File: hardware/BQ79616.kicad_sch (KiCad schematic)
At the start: 9 parts, among them CN7 4x100nF, IC2 BQ79616PAPR

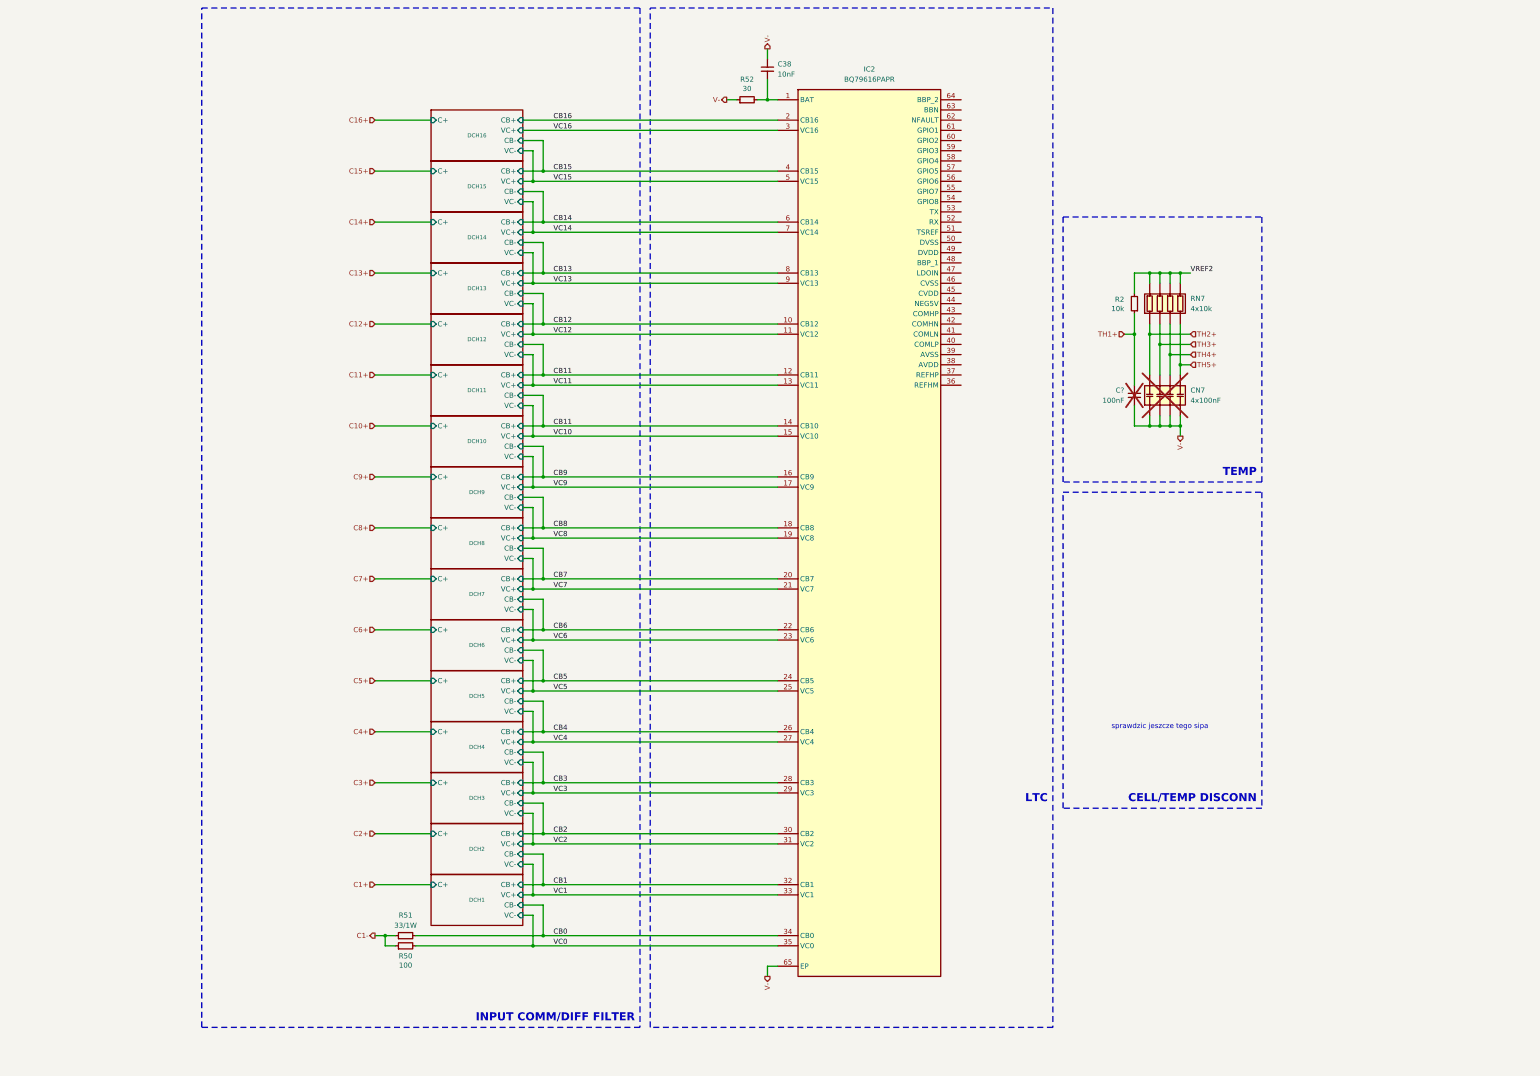
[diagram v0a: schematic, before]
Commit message: sync
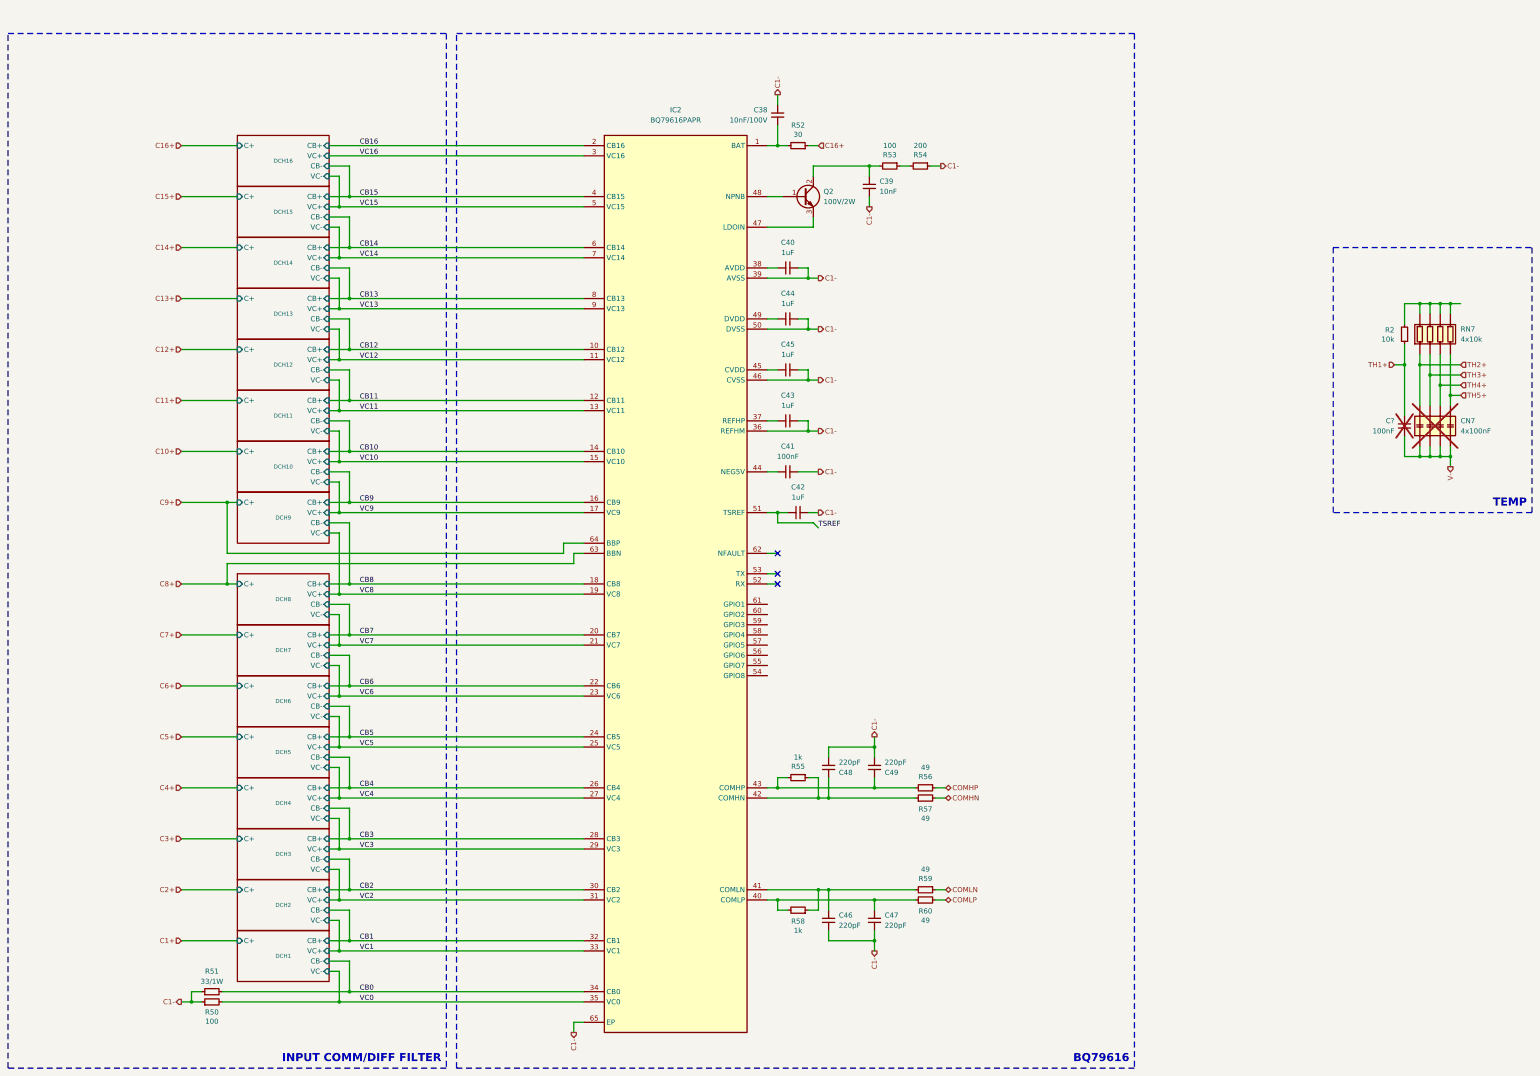
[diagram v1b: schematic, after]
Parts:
- added C39: 10nF, Capacitor_SMD:C_0603_1608Metric, symbol Device:C_Small
- added C40, C42, C43, C44, C45: 1uF, Capacitor_SMD:C_0603_1608Metric, symbol Device:C_Small
- added C41: 100nF, Capacitor_SMD:C_0603_1608Metric, symbol Device:C_Small
- added C46, C47, C48, C49: 220pF, Capacitor_SMD:C_0603_1608Metric, symbol Device:C_Small
- added Q2: 100V/2W, Package_TO_SOT_SMD:SOT-223-3_TabPin2, symbol Device:Q_NPN_BCE
- added R53: 100, Resistor_SMD:R_0603_1608Metric, symbol PUTM_EV_BMS_HV_Slave_2021-rescue:R_Small-Device
- added R54: 200, Resistor_SMD:R_0603_1608Metric, symbol PUTM_EV_BMS_HV_Slave_2021-rescue:R_Small-Device
- added R55, R58: 1k, Resistor_SMD:R_0603_1608Metric, symbol PUTM_EV_BMS_HV_Slave_2021-rescue:R_Small-Device
- added R56, R57, R59, R60: 49, Resistor_SMD:R_0603_1608Metric, symbol PUTM_EV_BMS_HV_Slave_2021-rescue:R_Small-Device
- C38: value 10nF -> 10nF/100V
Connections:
- net C1-: now also C38.1, IC2.36 (REFHM), IC2.39 (AVSS), IC2.46 (CVSS), IC2.50 (DVSS), IC2.65 (EP), C39.2, C40.2, C41.2, C42.2, C43.2, C44.2, C45.2, C46.2, C47.2, C48.2, C49.2, R54.1
- net C16+: now also R52.1
- net C8+: now also IC2.63 (BBN)
- net C9+: now also IC2.64 (BBP)
- net CB11: no longer IC2.14 (CB10)
- net V-: no longer C38.1, IC2.65 (EP), R52.1
- net at IC2.37 (REFHP): now also C43.1
- net at IC2.38 (AVDD): now also C40.1
- net at IC2.40 (COMLP): now also C47.1, R58.2, R60.1
- net at IC2.41 (COMLN): now also C46.1, R58.1, R59.2
- net at IC2.42 (COMHN): now also C48.1, R55.1, R57.1
- net at IC2.43 (COMHP): now also C49.1, R55.2, R56.2
- net at IC2.44 (NEG5V): now also C41.1
- net at IC2.45 (CVDD): now also C45.1
- net at IC2.47 (LDOIN): now also Q2.3 (E)
- net at IC2.48 (NPNB): now also Q2.1 (B)
- net at IC2.49 (DVDD): now also C44.1
- net TSREF: now reaches IC2.51 (TSREF)
- net TSREF: now also C42.1
- net VREF2: no longer names the net of R2.2, RN7.5 (R4.2), RN7.6 (R3.2), RN7.7 (R2.2), RN7.8 (R1.2)
- new net: C39.1, Q2.2 (C), R53.2
- new net: R53.1, R54.2
- new net CB10: IC2.14 (CB10)
- new net COMHN: R57.2
- new net COMHP: R56.1
- new net COMLN: R59.1
- new net COMLP: R60.2
- no-connect marks 0 -> 3
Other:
- note added: "BQ79616"
- note removed: "CELL/TEMP DISCONN"
- note removed: "LTC"
- note removed: "sprawdzic jeszcze tego sipa"
- moved on the sheet: C38, C?, CN7, IC2, R2, R50, R51, R52, RN7
